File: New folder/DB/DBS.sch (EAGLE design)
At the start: 58 parts, among them J1 TYPE-C-31-M-12, J10 TYPE-C-31-M-12, J11 TYPE-C-31-M-12, J12 TYPE-C-31-M-12, J13 TYPE-C-31-M-12, J14 TYPE-C-31-M-12, J15 TYPE-C-31-M-12, J16 TYPE-C-31-M-12, J17 TYPE-C-31-M-12, J18 TYPE-C-31-M-12, J19 TYPE-C-31-M-12, J20 TYPE-C-31-M-12, J21 TYPE-C-31-M-12, J22 TYPE-C-31-M-12, J23 TYPE-C-31-M-12, J24 TYPE-C-31-M-12, J25 TYPE-C-31-M-12, J26 TYPE-C-31-M-12, J3 TYPE-C-31-M-12, J4 TYPE-C-31-M-12, J5 TYPE-C-31-M-12, J6 TYPE-C-31-M-12, J7 TYPE-C-31-M-12, J8 TYPE-C-31-M-12, J9 TYPE-C-31-M-12, X1 SM04B-SRSS-TB, X10 SM04B-SRSS-TB, X11 SM04B-SRSS-TB, X12 SM04B-SRSS-TB, X13 SM04B-SRSS-TB, X14 SM04B-SRSS-TB, X15 SM04B-SRSS-TB, X16 SM04B-SRSS-TB, X17 SM04B-SRSS-TB, X18 SM04B-SRSS-TB, X19 SM04B-SRSS-TB, X20 SM04B-SRSS-TB, X21 SM04B-SRSS-TB, X22 SM04B-SRSS-TB, X23 SM04B-SRSS-TB, X24 SM04B-SRSS-TB, X25 SM04B-SRSS-TB, X26 SM04B-SRSS-TB, X3 SM04B-SRSS-TB, X4 SM04B-SRSS-TB, X5 SM04B-SRSS-TB, X6 SM04B-SRSS-TB, X7 SM04B-SRSS-TB, X8 SM04B-SRSS-TB, X9 SM04B-SRSS-TB

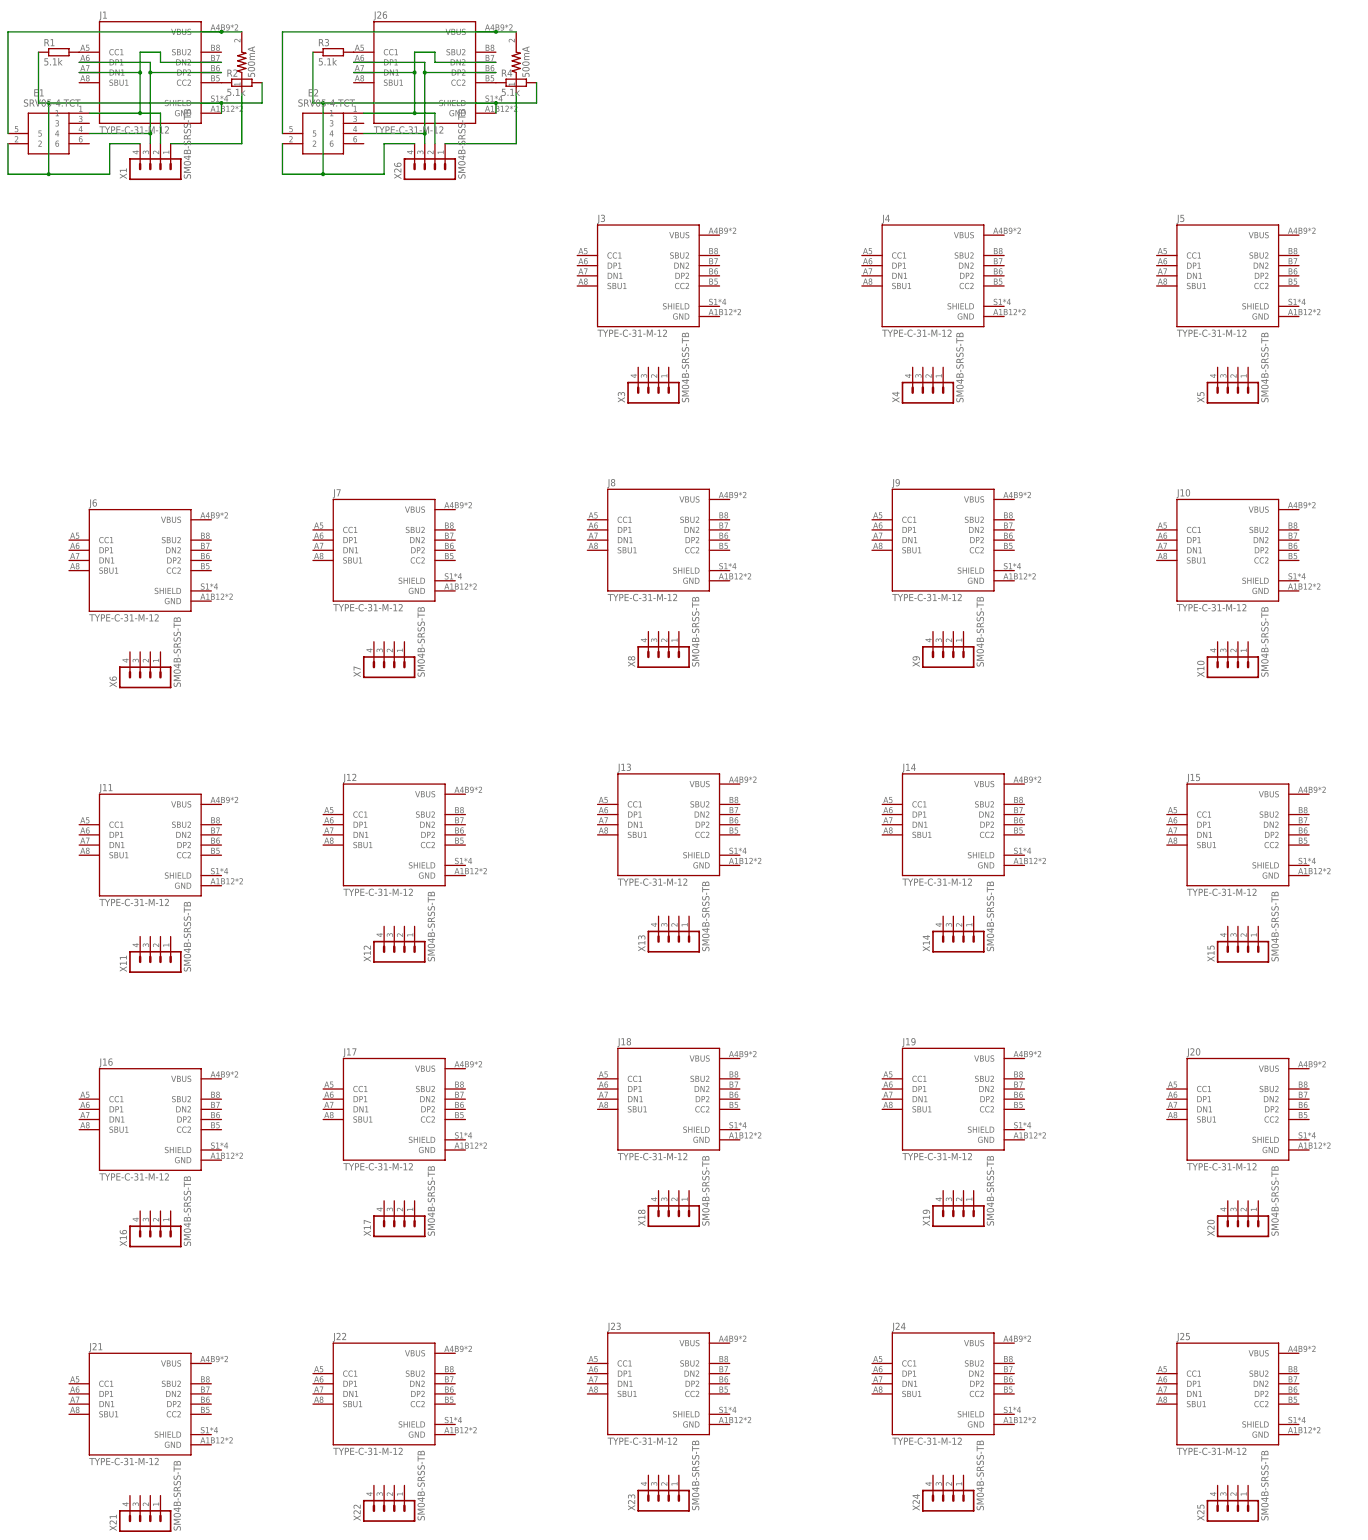
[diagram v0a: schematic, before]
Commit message: add
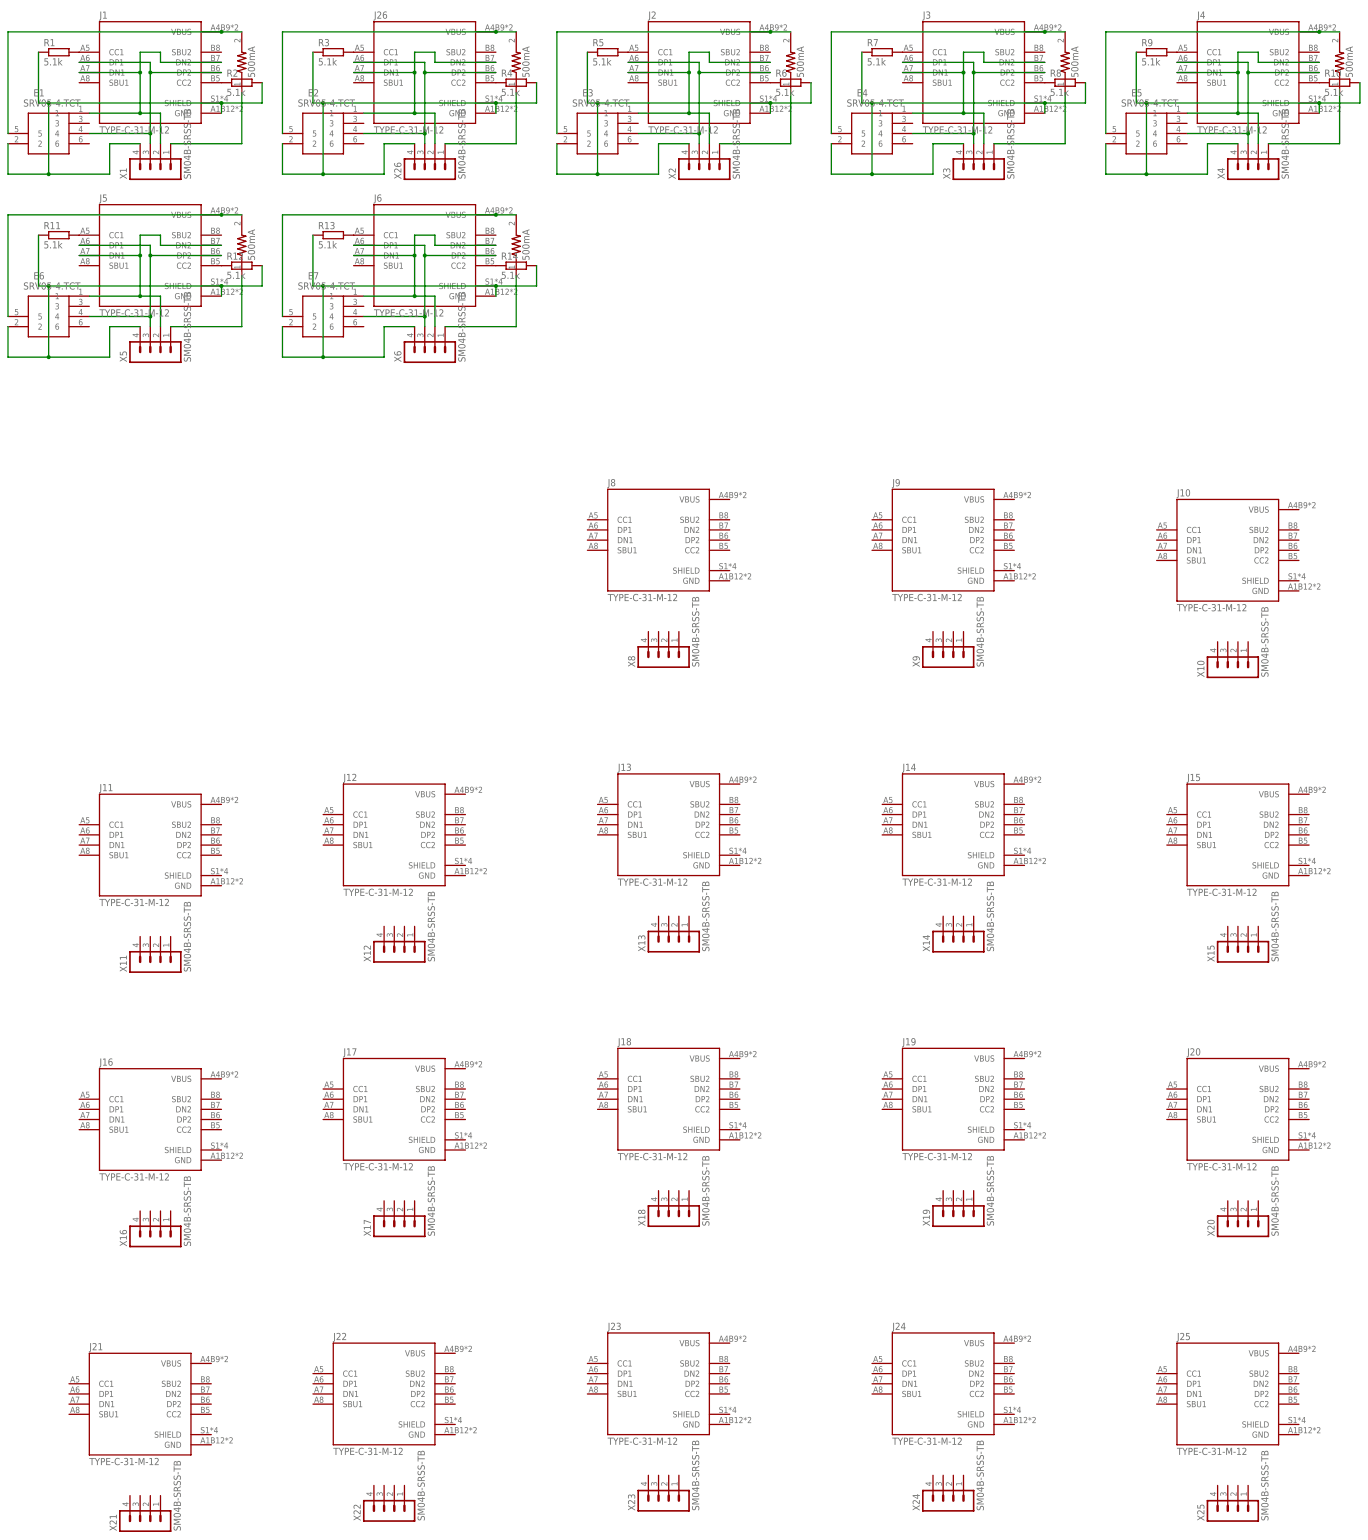
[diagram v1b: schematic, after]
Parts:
- removed J7: TYPE-C-31-M-12, TYPE-C-31-M-12:TYPE-C-31-M-12
- removed X7: SM04B-SRSS-TB, con-JST SH:SM04B-SRSS-TB
- added E3, E4, E5, E6, E7: SRV05-4.TCT, SRV05-4.TCT:SRV05-4.TCT
- added F3, F4, F5, F6, F7: 500mA, fuse:0ZCJ0075AF2E
- added J2: TYPE-C-31-M-12, TYPE-C-31-M-12:TYPE-C-31-M-12
- added R10, R11, R12, R13, R14, R5, R6, R7, R8, R9: 5.1k, Components:RESISTOR-0603
- added X2: SM04B-SRSS-TB, con-JST SH:SM04B-SRSS-TB
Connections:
- new net DN3: E3.1, J2.DN1, J2.DN2, X2.2
- new net DN4: E4.1, J3.DN1, J3.DN2, X3.2
- new net DN5: E5.1, J4.DN1, J4.DN2, X4.2
- new net DN6: E6.1, J5.DN1, J5.DN2, X5.2
- new net DN7: E7.1, J6.DN1, J6.DN2, X6.2
- new net DP3: E3.4, J2.DP1, J2.DP2, X2.3
- new net DP4: E4.4, J3.DP1, J3.DP2, X3.3
- new net DP5: E5.4, J4.DP1, J4.DP2, X4.3
- new net DP6: E6.4, J5.DP1, J5.DP2, X5.3
- new net DP7: E7.4, J6.DP1, J6.DP2, X6.3
- new net GND1: E3.2, J2.GND, J2.SHIELD, R5.1, R6.2, X2.4
- new net GND2: E4.2, J3.GND, J3.SHIELD, R7.1, R8.2, X3.4
- new net GND3: E5.2, J4.GND, J4.SHIELD, R10.2, R9.1, X4.4
- new net GND4: E6.2, J5.GND, J5.SHIELD, R11.1, R12.2, X5.4
- new net GND5: E7.2, J6.GND, J6.SHIELD, R13.1, R14.2, X6.4
- new net N$105: E3.5, F3.2, J2.VBUS
- new net N$106: F3.1, X2.1
- new net N$107: J2.CC1, R5.2
- new net N$108: J2.CC2, R6.1
- new net N$109: E4.5, F4.2, J3.VBUS
- new net N$110: F4.1, X3.1
- new net N$111: J3.CC1, R7.2
- new net N$112: J3.CC2, R8.1
- new net N$113: E5.5, F5.2, J4.VBUS
- new net N$114: F5.1, X4.1
- new net N$115: J4.CC1, R9.2
- new net N$116: J4.CC2, R10.1
- new net N$117: E6.5, F6.2, J5.VBUS
- new net N$118: F6.1, X5.1
- new net N$119: J5.CC1, R11.2
- new net N$120: J5.CC2, R12.1
- new net N$121: E7.5, F7.2, J6.VBUS
- new net N$122: F7.1, X6.1
- new net N$123: J6.CC1, R13.2
- new net N$124: J6.CC2, R14.1
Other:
- moved on the sheet: J3, J4, J5, J6, X3, X4, X5, X6
